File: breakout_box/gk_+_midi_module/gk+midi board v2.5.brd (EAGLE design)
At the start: 65.2 x 100 mm, 114 parts, among them T1 2N2222, T2 2N2222, U2 LMV324, U3 TLV2170DGKT, U4 L78LXX, U5 MIC5205-3.3, U6 MSP430G2553RHB32, X1 QUARZ5

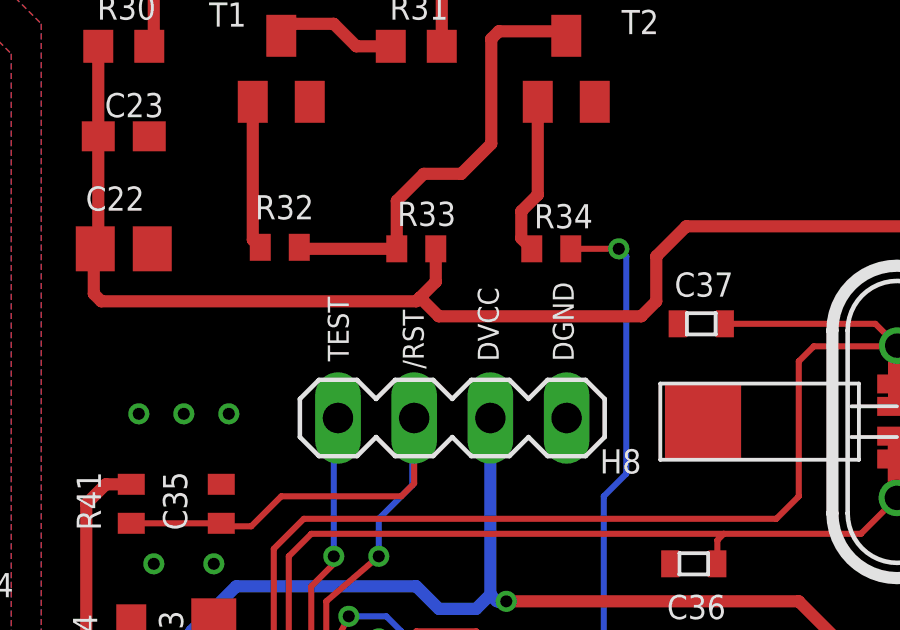
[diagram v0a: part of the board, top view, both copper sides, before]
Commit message: updates
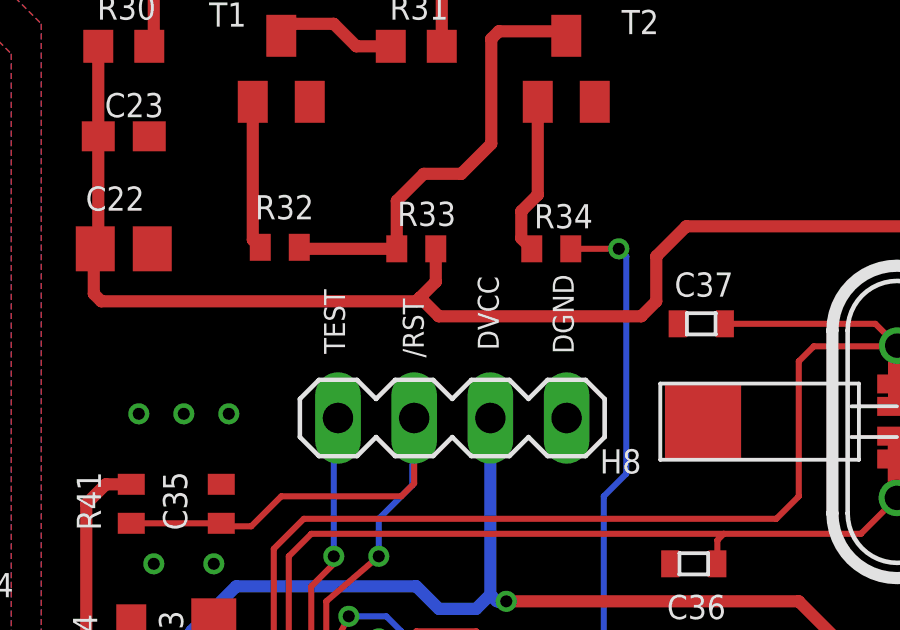
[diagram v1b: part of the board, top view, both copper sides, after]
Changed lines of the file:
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@@
 <text x="54.5" y="19.75" size="0.7" layer="25" font="vector" ratio="12">GND</text>
 <text x="59.75" y="19.75" size="0.7" layer="25" font="vector" ratio="12">GND</text>
-<text x="40.75" y="72.25" size="0.7" layer="25" font="vector" ratio="12" rot="R90">TEST</text>
-<text x="43.25" y="72" size="0.7" layer="25" font="vector" ratio="12" rot="R90">/RST</text>
-<text x="45.75" y="72.25" size="0.7" layer="25" font="vector" ratio="12" rot="R90">DVCC</text>
-<text x="48.25" y="72.25" size="0.7" layer="25" font="vector" ratio="12" rot="R90">DGND</text>
+<text x="40.625" y="72.5" size="0.7" layer="25" font="vector" ratio="12" rot="R90">TEST</text>
+<text x="43.25" y="72.375" size="0.7" layer="25" font="vector" ratio="12" rot="R90">/RST</text>
+<text x="45.75" y="72.625" size="0.7" layer="25" font="vector" ratio="12" rot="R90">DVCC</text>
+<text x="48.25" y="72.5" size="0.7" layer="25" font="vector" ratio="12" rot="R90">DGND</text>
 <text x="48" y="27.25" size="0.7" layer="25" font="vector" ratio="12">P1.1</text>
 <text x="48" y="29.75" size="0.7" layer="25" font="vector" ratio="12">P3.1</text>
